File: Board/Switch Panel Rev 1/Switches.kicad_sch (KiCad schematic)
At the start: 8 parts

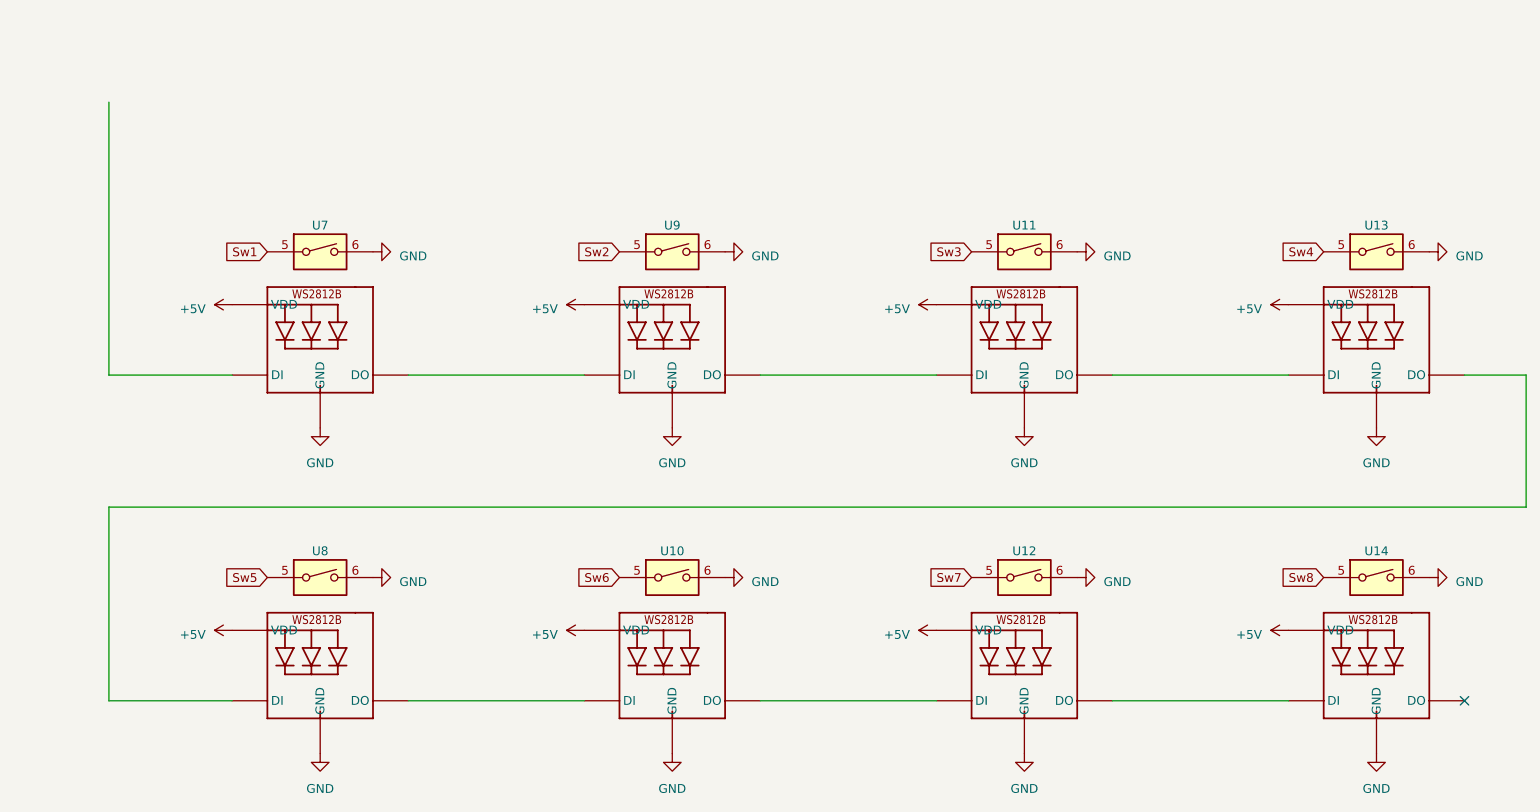
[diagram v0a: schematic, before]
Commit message: Board work
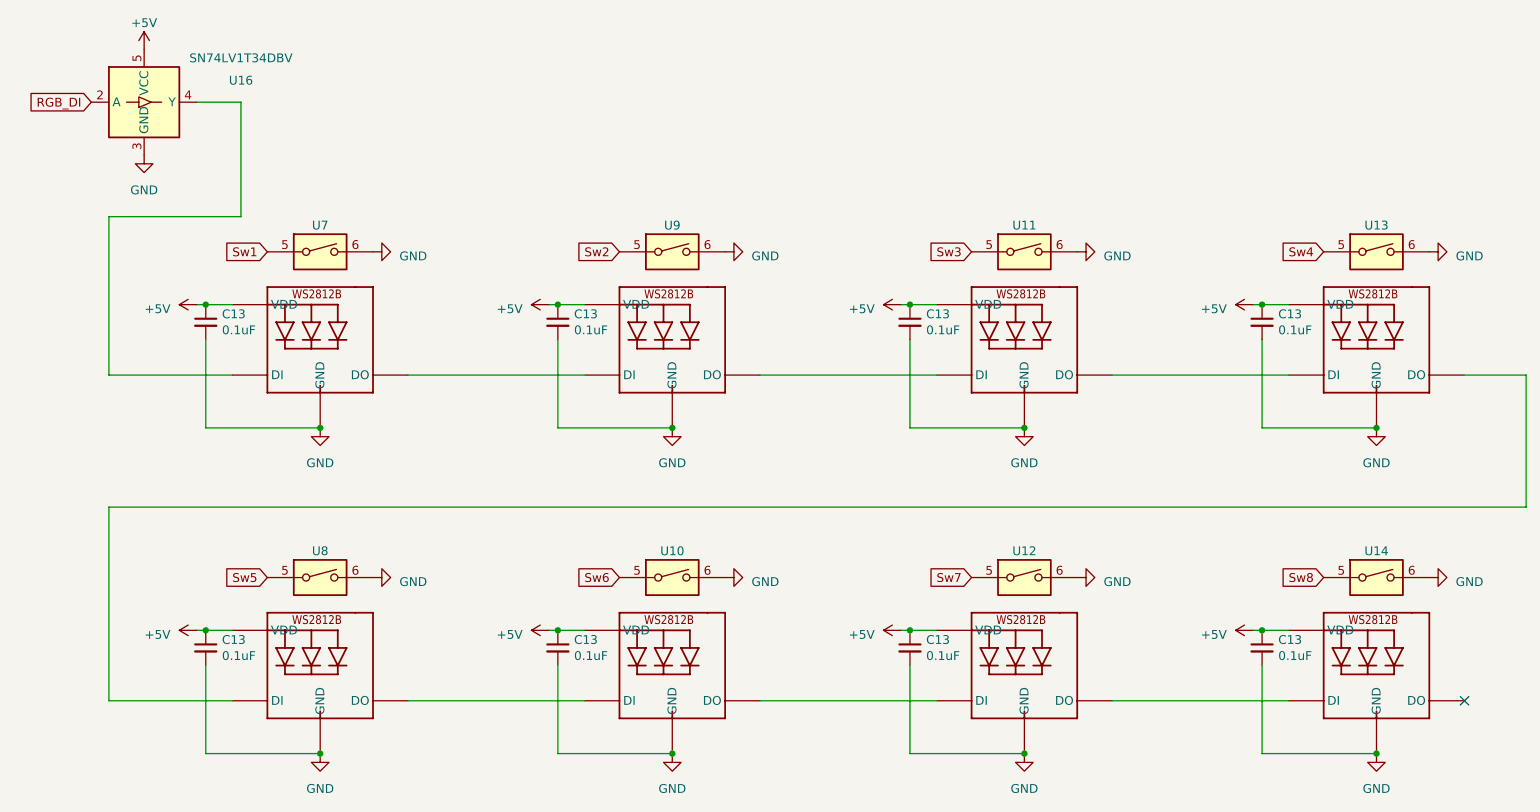
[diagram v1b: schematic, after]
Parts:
- added C13 (x8): 0.1uF, Capacitor_SMD:C_0603_1608Metric_Pad1.08x0.95mm_HandSolder, symbol Device:C_Small
- added U16: SN74LV1T34DBV, Package_TO_SOT_SMD:SOT-23-5, symbol Logic_LevelTranslator:SN74LV1T34DBV
- U10, U11, U12, U13, U14, U7, U8, U9: footprint MyKiCadLibraries:SW_Cherry_MX_Plate_RGB -> MyKiCadLibraries:SW_Kailh_Choc_RGB; symbol MyLibrary:Cherry_Mx_Rgb -> MyLibrary:Kailh_Choc_Rgb
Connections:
- net +5V: now also C13.1, C13.1, C13.1, C13.1, C13.1, C13.1, C13.1, C13.1, U16.5 (VCC)
- net GND: now also C13.2, C13.2, C13.2, C13.2, C13.2, C13.2, C13.2, C13.2, U16.3 (GND)
- net at U7.4 (DI): now also U16.4 (Y)
- new net RGB_DI: U16.2 (A)
